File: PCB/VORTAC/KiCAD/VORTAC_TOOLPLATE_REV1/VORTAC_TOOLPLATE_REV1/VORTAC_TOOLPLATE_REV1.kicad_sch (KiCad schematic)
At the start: 7 parts, among them J1 Conn_01x07, J2 Conn_01x02, J3 Conn_01x05

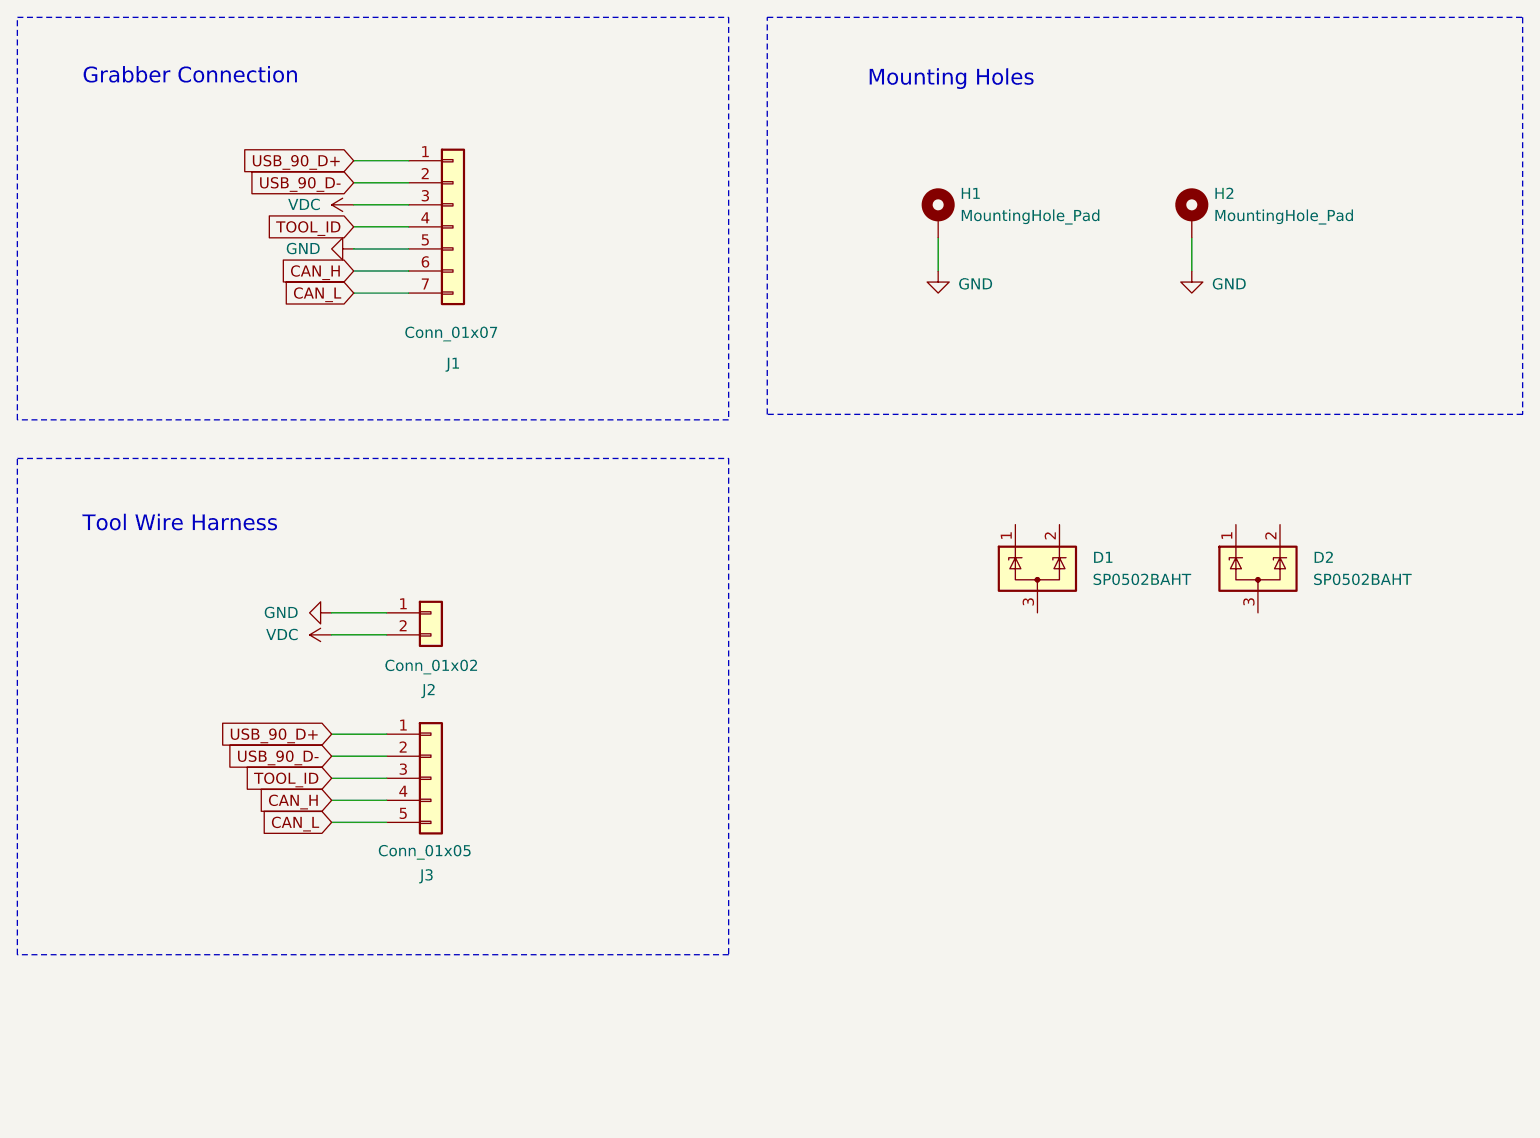
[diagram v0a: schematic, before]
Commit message: KONGSTRONG
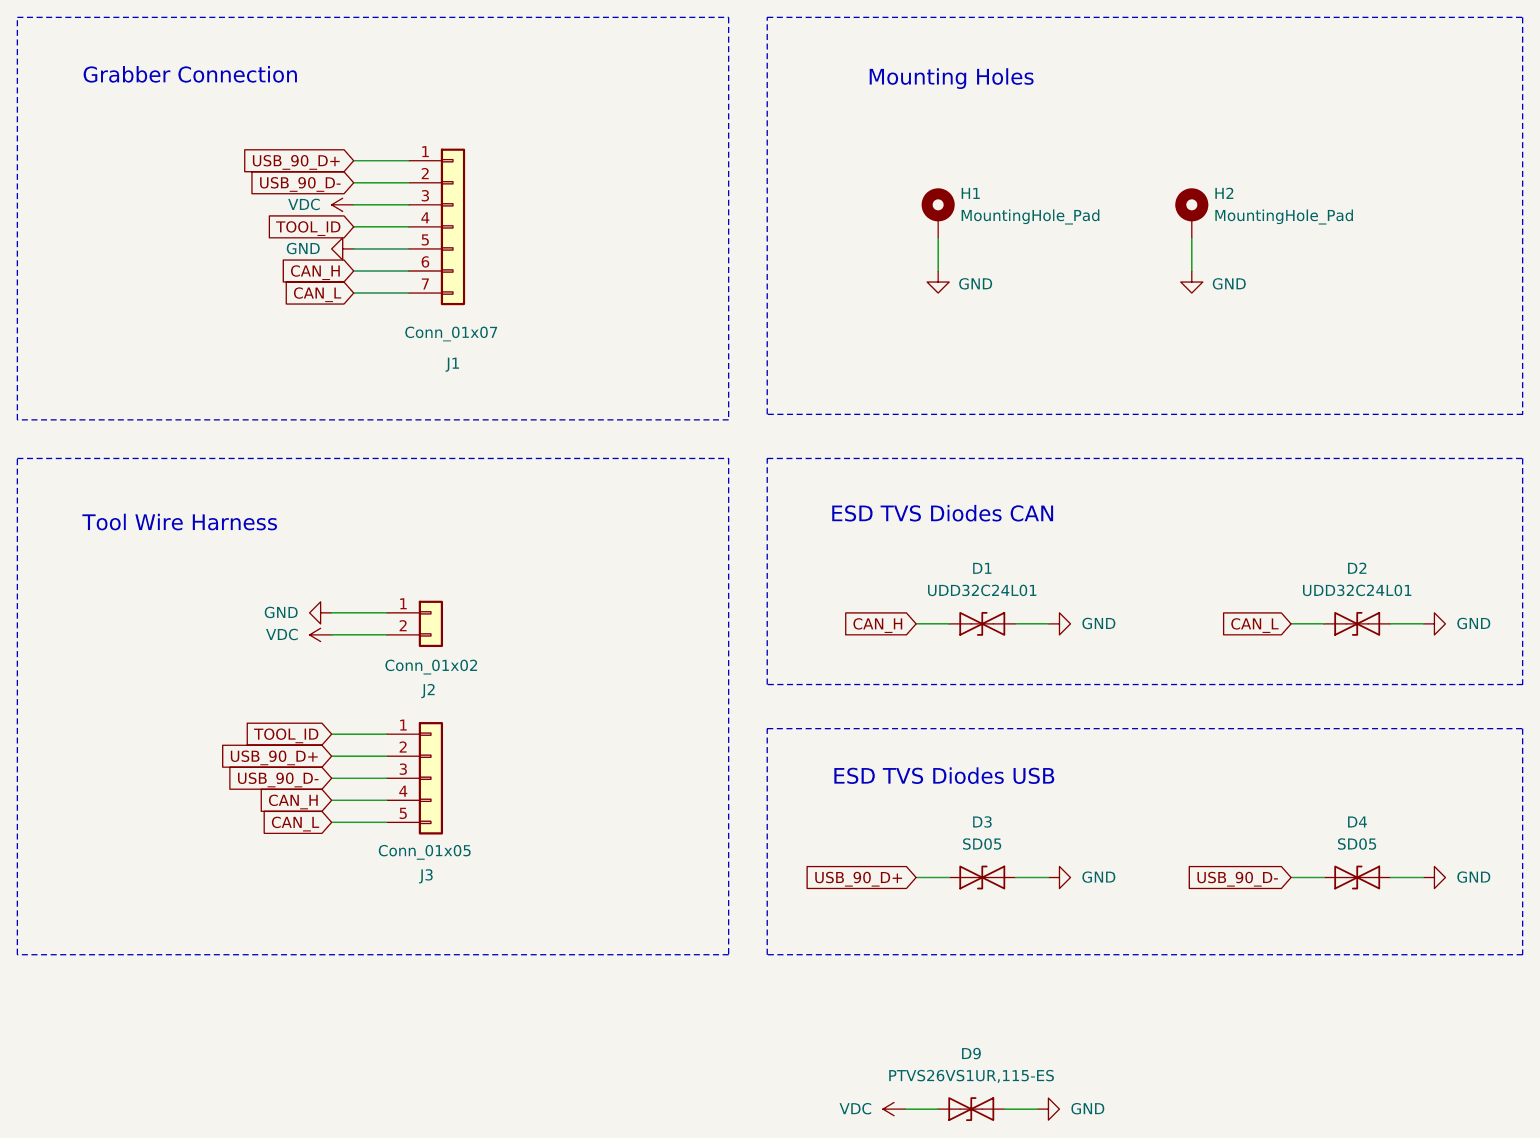
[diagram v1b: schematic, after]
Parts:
- removed D1, D2: SP0502BAHT, Package_TO_SOT_SMD:SOT-23, symbol Power_Protection:SP0502BAHT
- added D1, D2: UDD32C24L01, Diode_SMD:D_SOD-323, symbol Diode:SD24_SOD323
- added D3, D4: SD05, Diode_SMD:D_SOD-323, symbol Diode:SD24_SOD323
- added D9: PTVS26VS1UR,115-ES, Diode_SMD:D_SOD-123F, symbol Diode:SD24_SOD323
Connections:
- net CAN_H: now also D1.2 (A2)
- net CAN_L: now also D2.2 (A2)
- net GND: now also D1.1 (A1), D2.1 (A1), D3.1 (A1), D4.1 (A1), D9.1 (A1)
- net TOOL_ID: now also J3.1 (Pin_1); no longer J3.3 (Pin_3)
- net USB_90_D+: now also J3.2 (Pin_2), D3.2 (A2); no longer J3.1 (Pin_1)
- net USB_90_D-: now also J3.3 (Pin_3), D4.2 (A2); no longer J3.2 (Pin_2)
- net VDC: now also D9.2 (A2)
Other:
- note added: "ESD TVS Diodes CAN"
- note added: "ESD TVS Diodes USB"
